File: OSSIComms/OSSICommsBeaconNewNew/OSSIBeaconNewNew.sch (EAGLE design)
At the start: 116 parts, among them Q1 NX-3215, U1 ADL5530, U10 MCP1700_SOT23, U2 MAX890L, U3 NC7SZ04, U4 ADF7012, U5 MAX6369, U6 MSP430F2132, U7 OPA2347, U8 TPS3838, U9 MAX890L, X1 P-PAD-S, X2 ESQ-126-38-G-D, X3 P-PAD-S, X4 RFCON-MCX-R/A, X5 5268-02, X7 5268-03, X8 JTAG10PINMINI-H

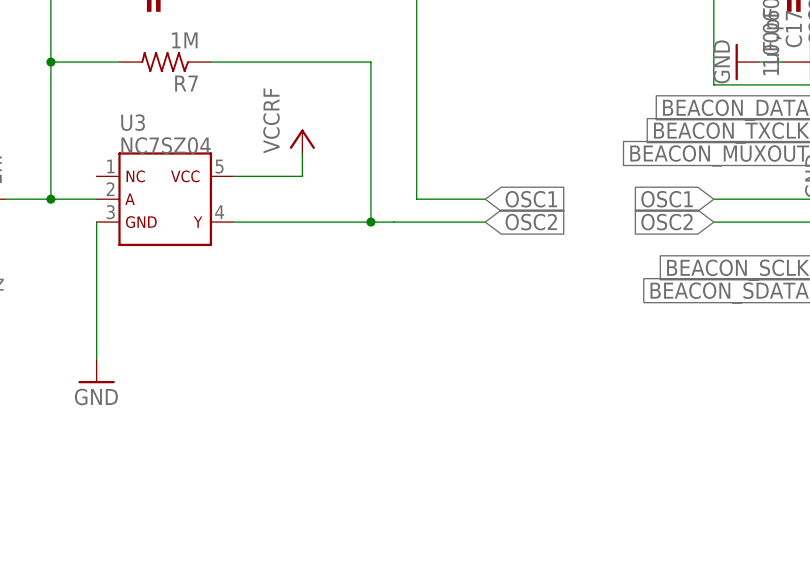
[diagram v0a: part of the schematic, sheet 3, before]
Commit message: comms names renumbred
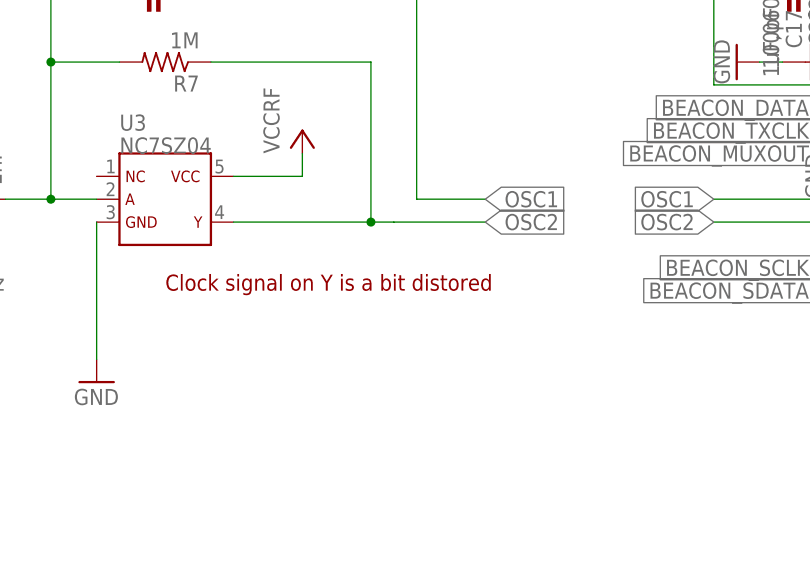
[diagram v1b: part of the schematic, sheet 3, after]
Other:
- note added: "Clock signal on Y is a bit distored"
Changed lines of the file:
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@@
 <plain>
 <text x="193.04" y="96.52" size="1.778" layer="94">tune L4 for for better PLL margin</text>
+<text x="86.36" y="106.68" size="1.778" layer="94">Clock signal on Y is a bit distored</text>
 </plain>
 <instances>
